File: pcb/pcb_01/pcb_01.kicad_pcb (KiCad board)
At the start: 2 copper layers, 2 parts, among them J1 Screw_Terminal_01x02

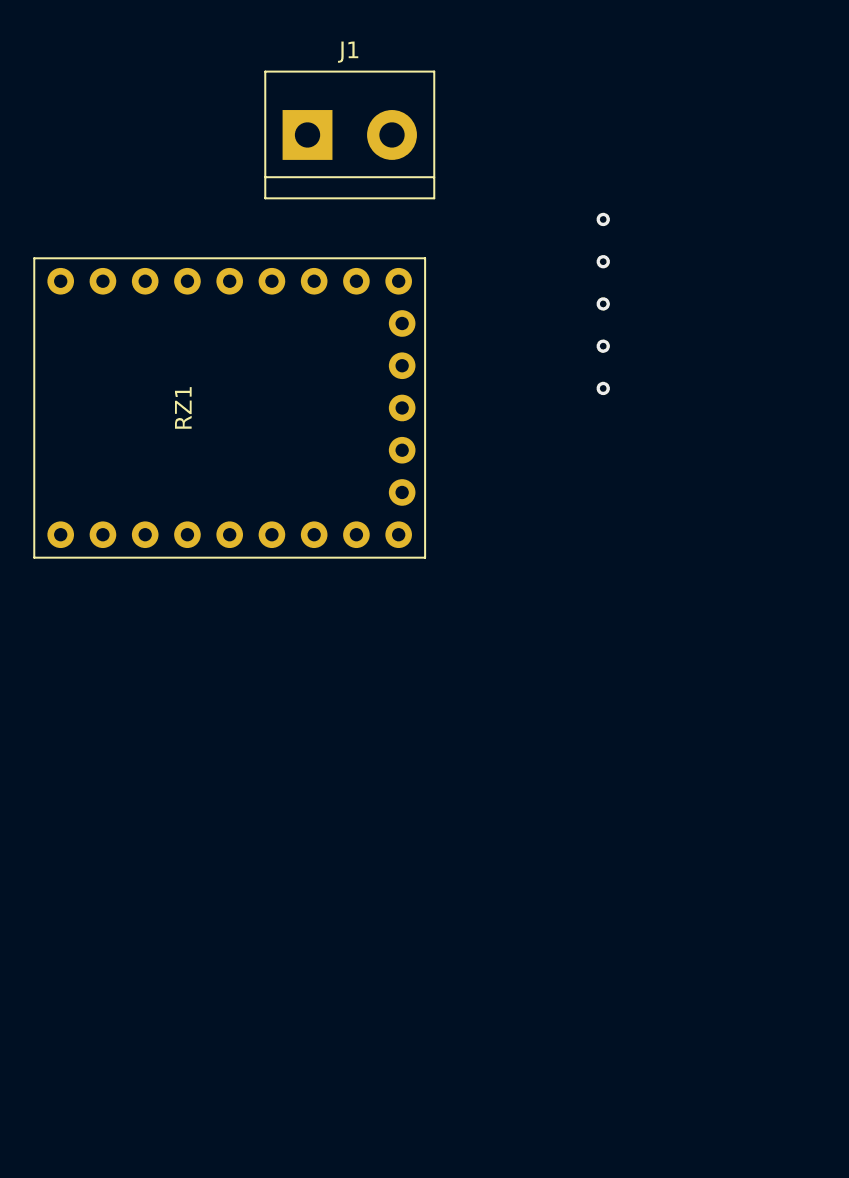
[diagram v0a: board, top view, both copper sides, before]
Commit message: update pcb
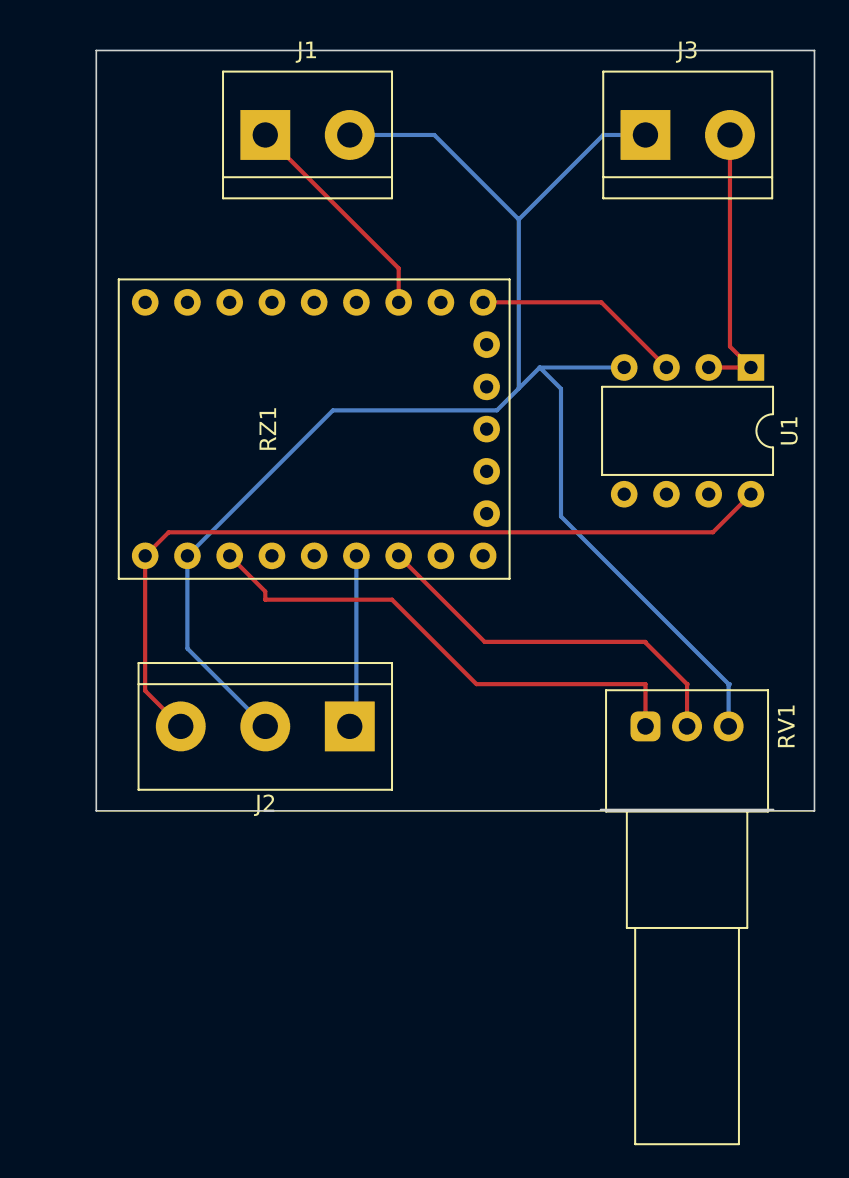
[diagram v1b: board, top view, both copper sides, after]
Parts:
- added J2: Screw_Terminal_01x03, TerminalBlock:TerminalBlock_bornier-3_P5.08mm, F.Cu at (127.0, 111.8)
- added J3: Screw_Terminal_01x02, TerminalBlock:TerminalBlock_bornier-2_P5.08mm, F.Cu at (144.8, 76.2)
- added RV1: R_Potentiometer, Potentiometer_THT:Potentiometer_Alps_RK097_Single_Horizontal, F.Cu at (144.8, 111.8)
- added U1: LM358, Package_DIP:DIP-8_W7.62mm, F.Cu at (151.1, 90.2)
- moved RZ1 5.24 mm to (136.6, 102.9)
- moved J1 2.54 mm to (121.9, 76.2)
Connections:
- J1 pad 1: Net-(RZ1-Pad23) -> Net-(RZ1-Pad7)
- J1 pad 2: Net-(RZ1-Pad6) -> Net-(RZ1-Pad23)
- RZ1 pad 17: unconnected-(RZ1-Pad17) -> Net-(RZ1-Pad17)
- RZ1 pad 18: unconnected-(RZ1-Pad18) -> Net-(RZ1-Pad18)
- RZ1 pad 21: unconnected-(RZ1-Pad21) -> Net-(RZ1-Pad21)
- RZ1 pad 22: unconnected-(RZ1-Pad22) -> Net-(RZ1-Pad22)
- RZ1 pad 6: Net-(RZ1-Pad6) -> unconnected-(RZ1-Pad6)
- RZ1 pad 7: unconnected-(RZ1-Pad7) -> Net-(RZ1-Pad7)
- RZ1 pad 9: unconnected-(RZ1-Pad9) -> Net-(RZ1-Pad9)
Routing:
- net Net-(RZ1-Pad23): track 0.00 -> 101.6 mm
- net Net-(RZ1-Pad22): track 0.00 -> 49.1 mm
- net Net-(RZ1-Pad21): track 0.00 -> 31.0 mm
- net Net-(RZ1-Pad17): track 0.00 -> 23.1 mm
- net Net-(U1-Pad1): track 0.00 -> 17.0 mm
- net Net-(RZ1-Pad7): track 0.00 -> 13.4 mm
- net Net-(RZ1-Pad9): track 0.00 -> 12.6 mm
- net Net-(RZ1-Pad18): track 0.00 -> 10.4 mm
- net (no net): vias 5 -> 0
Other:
- board outline added: 43.2 x 45.7 mm
